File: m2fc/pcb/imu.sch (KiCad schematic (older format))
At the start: 50 parts, among them IC301 ADXL375, IC302 ADXL345, IC303 MS5611-01BA03, IC304 HMC5883L, IC305 L3G4200D

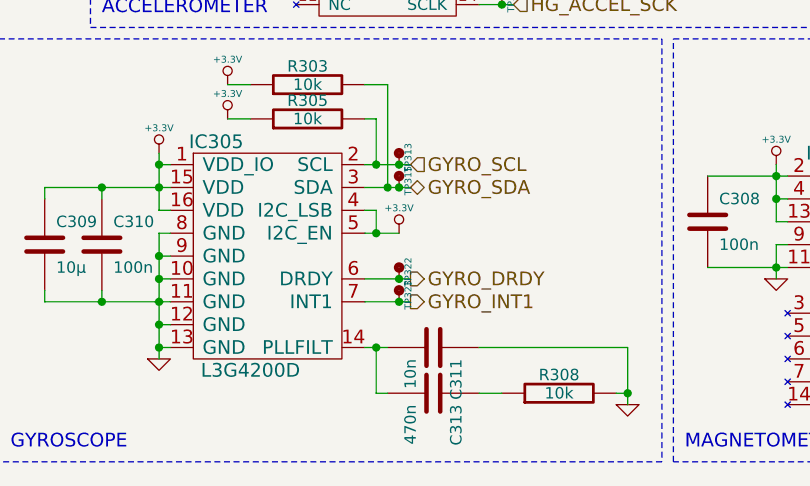
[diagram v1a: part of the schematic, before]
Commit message: routing continues
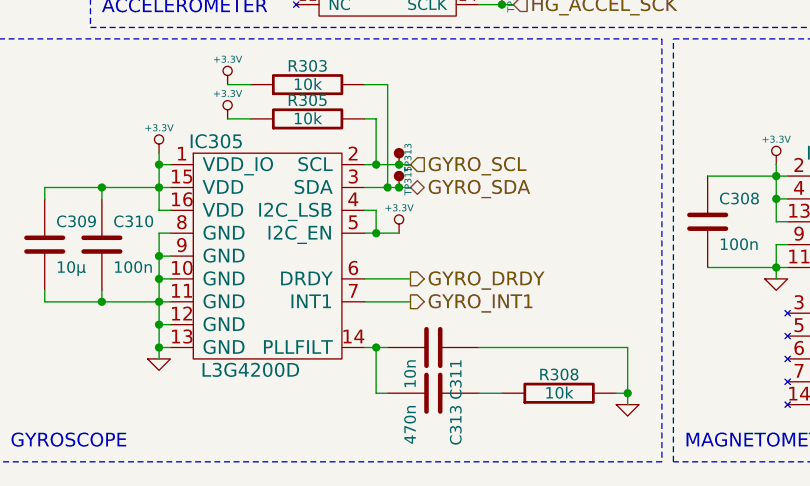
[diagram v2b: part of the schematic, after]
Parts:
- removed TP322, TP323: TESTPAD, m2fc:TESTPAD, symbol TESTPAD
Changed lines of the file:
@@
-	0    -1   -1   0
-$EndComp
-$Comp
-L TESTPAD TP322
-U 1 1 53B7FC94
-P 3950 4450
-F 0 "TP322" H 3980 4410 30  0000 C CNN
-F 1 "TESTPAD" H 3950 4500 60  0001 C CNN
-F 2 "m2fc:TESTPAD" H 3950 4450 60  0001 C CNN
-F 3 "" H 3950 4450 60  0000 C CNN
-	1    3950 4450
 	0    -1   -1   0
 $EndComp
 Connection ~ 3950 4050
 Connection ~ 3950 3950
-Connection ~ 3950 4450
 $Comp
 L TESTPAD TP314
@@
 Wire Wire Line
 	3800 4550 4000 4550
-$Comp
-L TESTPAD TP323
-U 1 1 53C45860
-P 3950 4550
-F 0 "TP323" H 3980 4510 30  0000 C CNN
-F 1 "TESTPAD" H 3950 4600 60  0001 C CNN
-F 2 "m2fc:TESTPAD" H 3950 4550 60  0001 C CNN
-F 3 "" H 3950 4550 60  0000 C CNN
-	1    3950 4550
-	0    -1   -1   0
-$EndComp
-Connection ~ 3950 4550
 Wire Wire Line
 	3800 4150 3850 4150
